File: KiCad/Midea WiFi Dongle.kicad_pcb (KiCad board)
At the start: 4 copper layers, 20 x 48.5 mm, 21 parts, among them J1 USB_A, Q1 BSS138, Q2 BSS138, SW1 PRG, SW2 RST, U1 LM1117-3.3, U2 ESP-12F

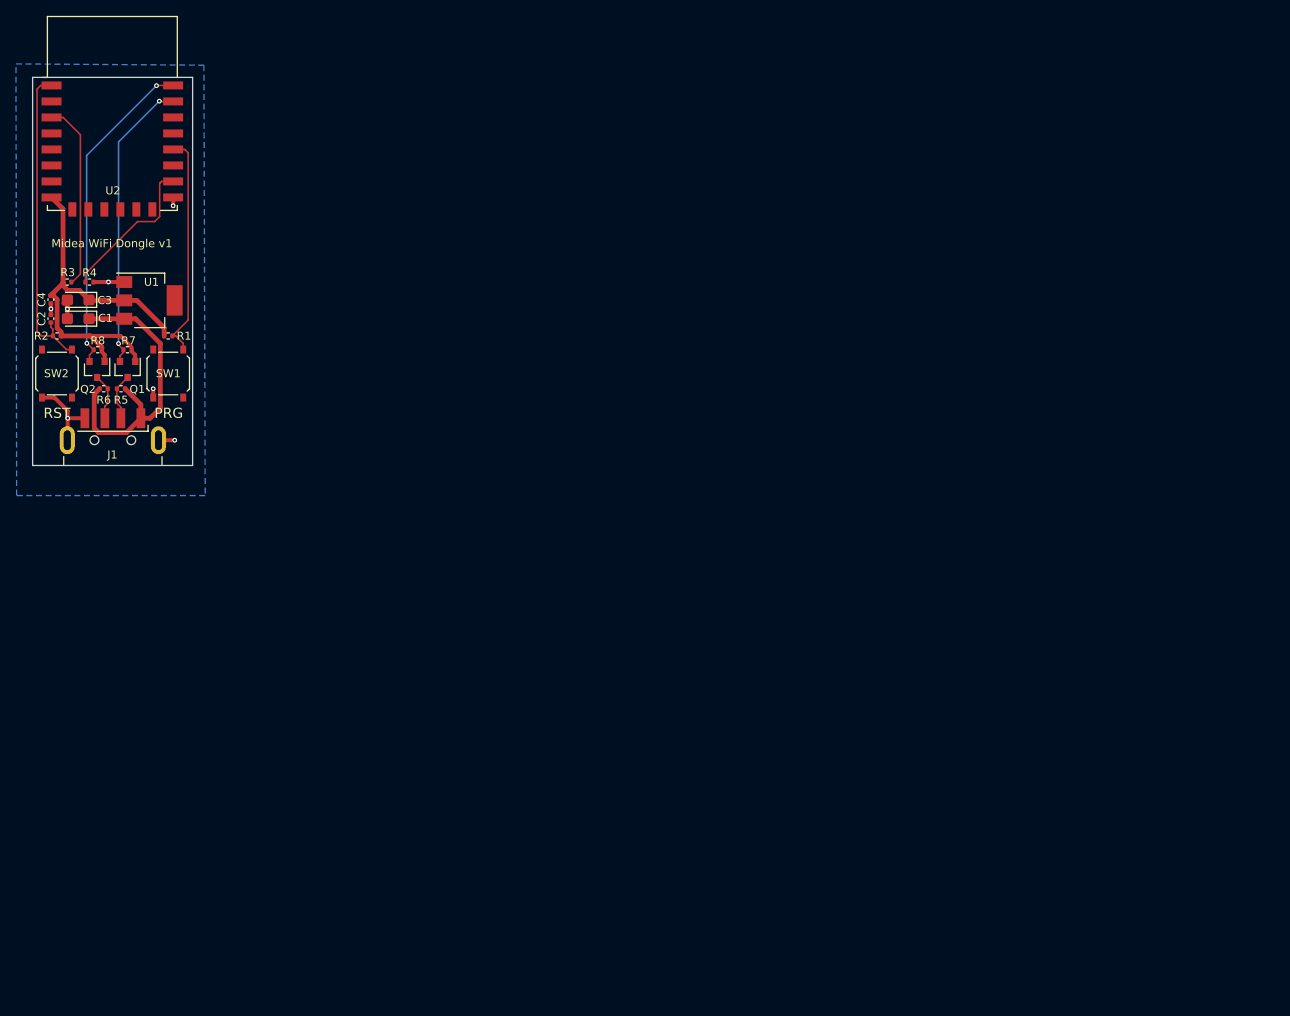
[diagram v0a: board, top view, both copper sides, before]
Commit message: Rework pcb and component sleection
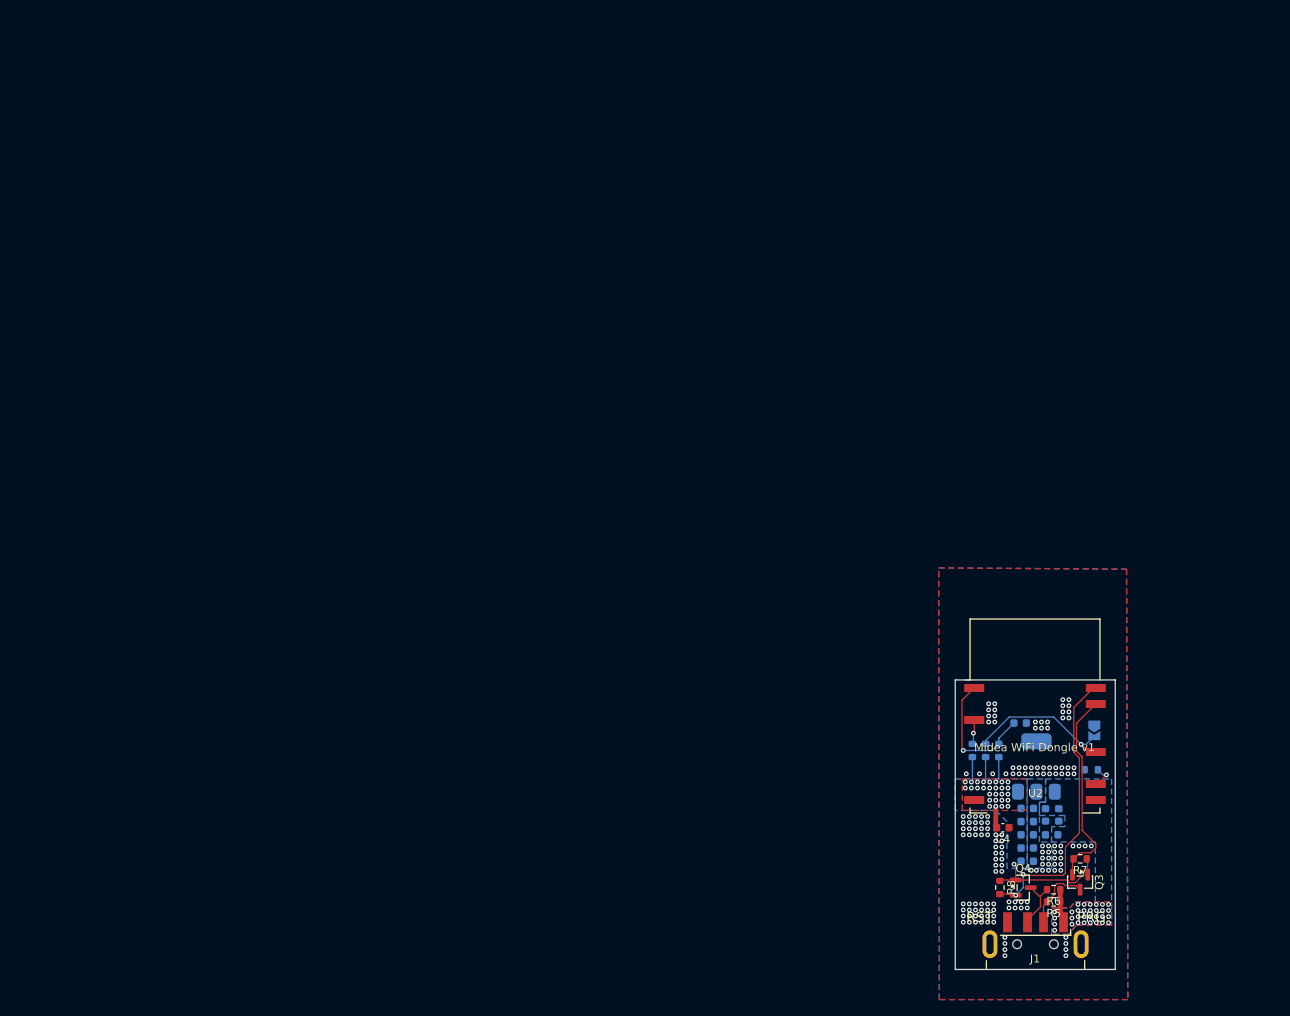
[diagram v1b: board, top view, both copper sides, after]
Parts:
- removed C1, C3: 47uF, Capacitor_Tantalum_SMD:CP_EIA-3216-10_Kemet-I
- removed Q1, Q2: BSS138, Package_TO_SOT_SMD:SOT-23
- removed REF**: KiCad-Logo2_5mm_SilkScreen, Symbol:KiCad-Logo2_5mm_SilkScreen
- removed REF**: OSHW-Logo2_14.6x12mm_SilkScreen, Symbol:OSHW-Logo2_14.6x12mm_SilkScreen
- removed SW1: PRG, mine:TS1187AXXX
- removed SW2: RST, mine:TS1187AXXX
- removed U1: LM1117-3.3, Package_TO_SOT_SMD:SOT-223
- added C10: 10u, Capacitor_SMD:C_0603_1608Metric, B.Cu at (160.5, 96.4)
- added C11: 10u, Capacitor_SMD:C_0603_1608Metric, B.Cu at (162.8, 92.3)
- added C12: 10u, Capacitor_SMD:C_0603_1608Metric, B.Cu at (164.5, 92.3)
- added C13: 10u, Capacitor_SMD:C_0603_1608Metric, B.Cu at (163.6, 94.7)
- added C5: 100nF, Capacitor_SMD:C_0603_1608Metric, B.Cu at (160.5, 91.4)
- added C6: 100nF, Capacitor_SMD:C_0603_1608Metric, B.Cu at (160.5, 98.0)
- added C8: 10u, Capacitor_SMD:C_0603_1608Metric, B.Cu at (160.5, 93.1)
- added C9: 10u, Capacitor_SMD:C_0603_1608Metric, B.Cu at (160.5, 94.7)
- added JP1: PROG, Jumper:SolderJumper-2_P1.3mm_Open_TrianglePad1.0x1.5mm, B.Cu at (168.9, 81.7)
- added Q3: AO3400A, Package_TO_SOT_SMD:SOT-23, F.Cu at (167.1, 100.7)
- added Q4: AO3400A, Package_TO_SOT_SMD:SOT-23, F.Cu at (160.0, 101.3)
- added U3: MCP1826S, Package_TO_SOT_SMD:SOT-223-3_TabPin2, B.Cu at (161.7, 86.2)
- C2: value 470uF -> 470pF; footprint Capacitor_SMD:C_0402_1005Metric -> Capacitor_SMD:C_0603_1608Metric; moved to B.Cu
- C4: footprint Capacitor_SMD:C_0402_1005Metric -> Capacitor_SMD:C_0603_1608Metric
- R1, R2, R3, R4: footprint Resistor_SMD:R_0402_1005Metric -> Resistor_SMD:R_0603_1608Metric; moved to B.Cu
- R5, R6, R7, R8: footprint Resistor_SMD:R_0402_1005Metric -> Resistor_SMD:R_0603_1608Metric
- moved R4 139.3 mm to (168.5, 86.6), turned to 180 degrees
- moved U2 137.7 mm to (161.5, 79.9)
- moved C4 136.1 mm to (157.5, 93.9), turned to 180 degrees
- moved R7 135.0 mm to (167.1, 97.7)
- moved R6 134.2 mm to (163.8, 101.6), turned to 180 degrees
- moved R5 133.1 mm to (163.8, 103.1)
- moved J1 131.4 mm to (161.6, 115.3)
- moved C2 131.3 mm to (159.6, 80.8), turned to 0 degrees
- moved R8 131.3 mm to (157.1, 101.3), turned to -90 degrees
- moved R2 128.6 mm to (157.0, 84.2), turned to -90 degrees
- moved R3 127.4 mm to (153.7, 84.2), turned to -90 degrees
- moved R1 114.6 mm to (155.3, 84.2), turned to -90 degrees
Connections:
- net +3V3 renamed +3.3V
- J1 pad 5: GND -> (no net)
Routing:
- net +5V: track 37.9 -> 4.16 mm, vias 0 -> 31
- net +3.3V: track 51.7 -> 28.0 mm, vias 0 -> 29
- net /RESET: track 39.5 -> 16.7 mm, vias 0 -> 1
- net GND: track 22.3 -> 0.00 mm, vias 7 -> 148
- net /EN: track 23.5 -> 3.08 mm, vias 0 -> 1
- net /GPIO15: track 19.4 -> 3.15 mm, vias 0 -> 1
- net /RX: track 36.8 -> 25.4 mm, vias 2 -> 0
- net /GPIO0: track 29.5 -> 19.3 mm, vias 0 -> 1
- net /TX: track 40.8 -> 35.9 mm
- net /TX_APPLIANCE: track 6.30 -> 8.98 mm
- net /RX_APPLIANCE: track 6.67 -> 7.45 mm
- added copper zone on B.Cu, net +3.3V
- added copper zone on F.Cu, net +3.3V
- added copper zone on B.Cu, net +5V
- added copper zone on F.Cu, net +5V
- added copper zone on F.Cu, net GND
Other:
- board size 20 x 48.5 mm -> 20 x 36.2 mm
- net class Default removed
- net class VCC removed

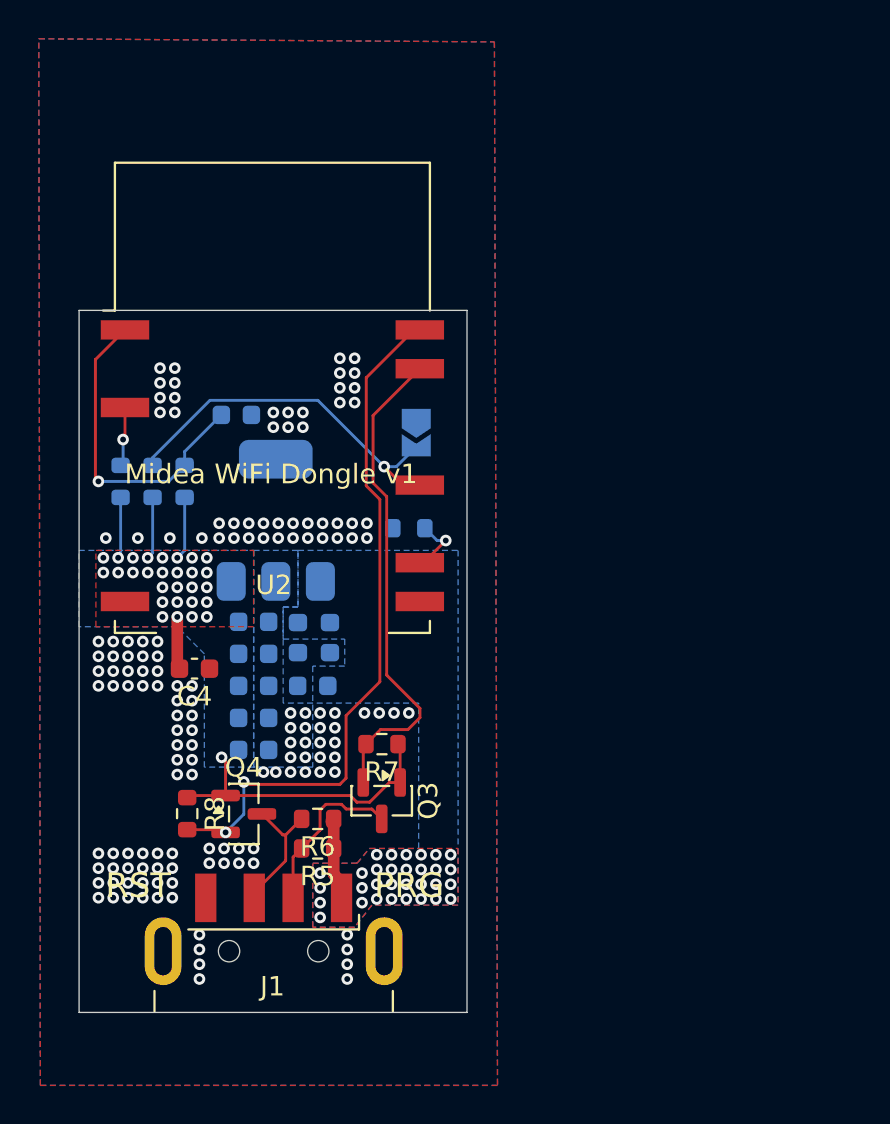
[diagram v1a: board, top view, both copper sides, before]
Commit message: Fix sinkscreen
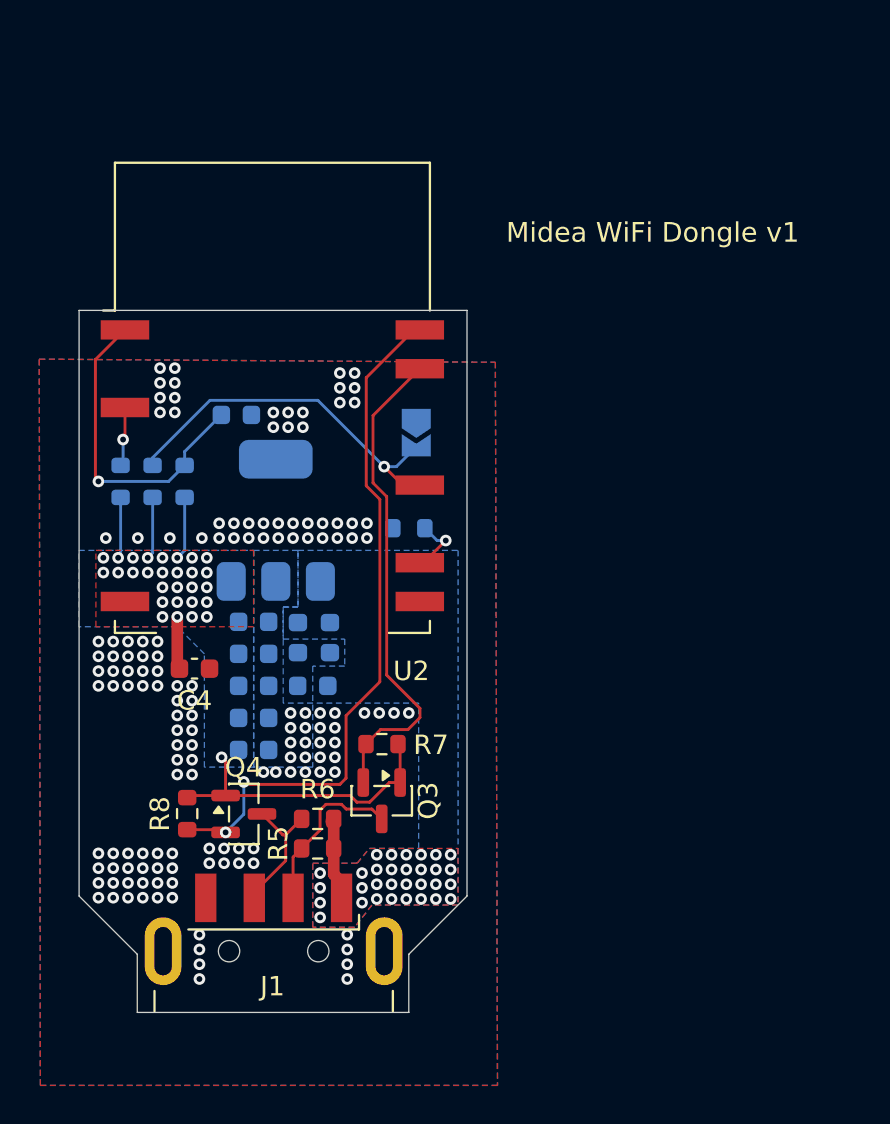
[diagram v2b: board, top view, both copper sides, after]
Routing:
- net GND: vias 148 -> 146
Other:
- outline, holes or cut-outs redrawn
- copper layers 4 -> 2
- board text added: "Copyright (C) 2026 René Klootwijk Alacrity Education"
- board text added: "MIDEA Dongle"
- board text added: "PROG"
- board text removed: "Copyright (C) 2020 René Klootwijk"
- board text removed: "PRG"
- board text removed: "RST"
